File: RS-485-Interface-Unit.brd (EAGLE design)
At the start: 53.4 x 30.4 mm, 16 parts, among them IC1 B0505S, IC2 ADM2483, IC3 78L05Z, X1 RJ11CONNECTOR, X2 RJ11CONNECTOR

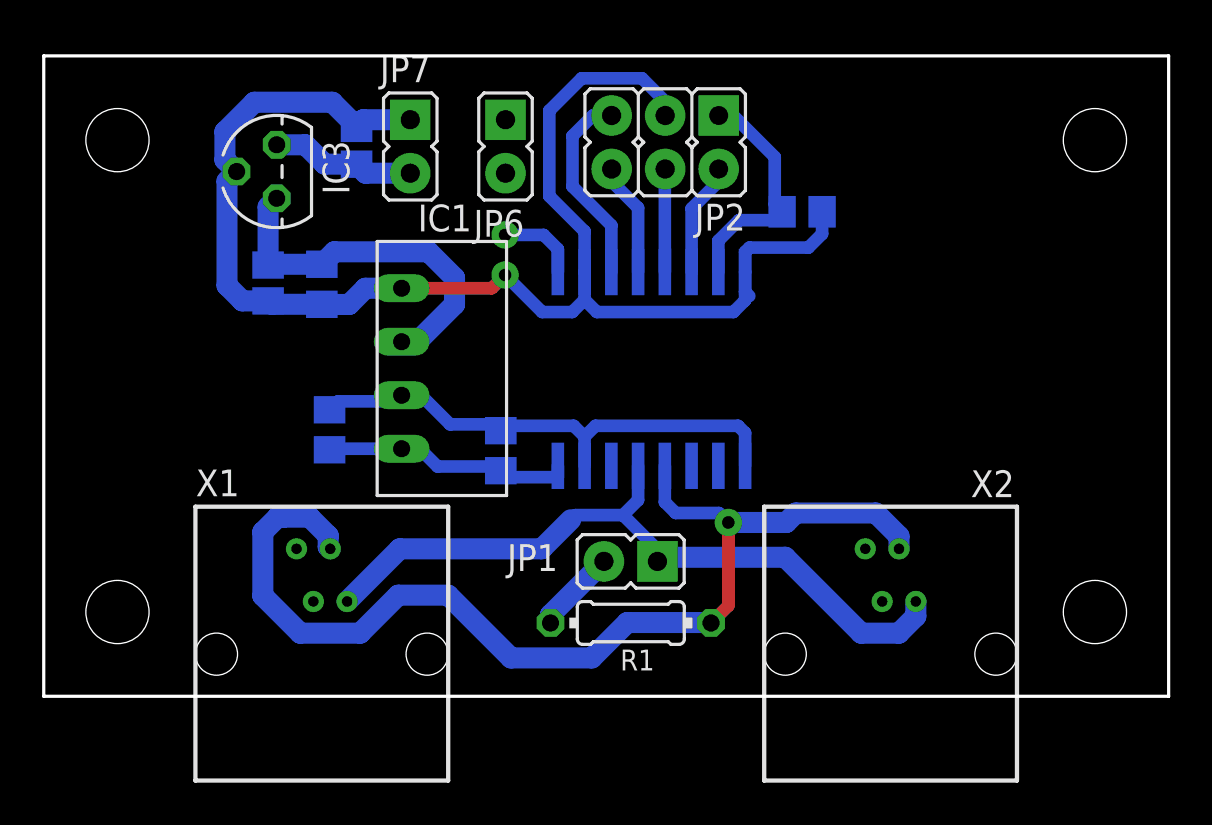
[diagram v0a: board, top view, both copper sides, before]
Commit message: Board tracing done
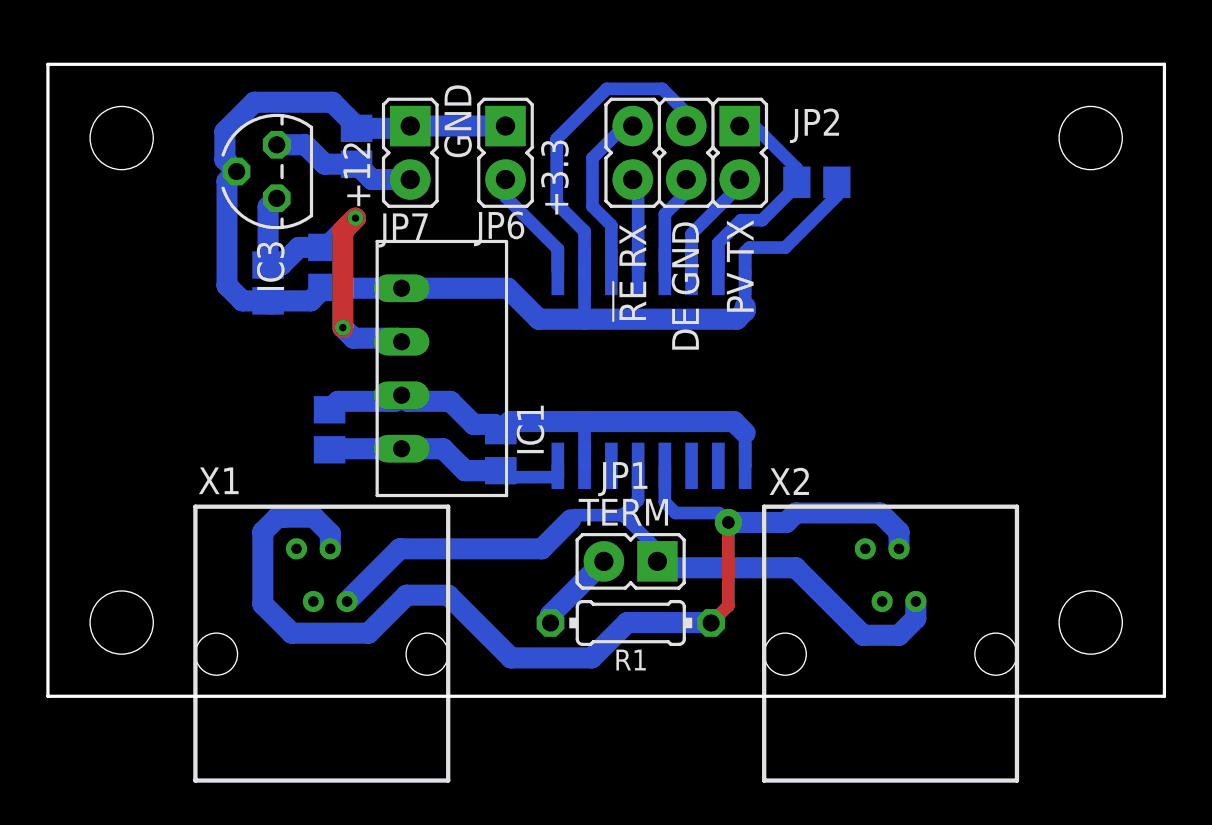
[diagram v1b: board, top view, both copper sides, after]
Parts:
- JP1: value (none) -> TERM
- moved R11 1.57 mm to (44.0, 31.0)
- moved JP2 1.12 mm to (37.8, 32.4)
- moved C2 0.81 mm to (20.6, 27.0)
- moved JP6 0.30 mm to (29.2, 32.4)
- moved JP7 0.30 mm to (24.7, 32.4)
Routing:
- net GND: track 69.4 -> 75.0 mm, vias 1 -> 0
- net VCCIO: track 12.0 -> 13.9 mm
- net +3V3: track 3.87 -> 5.42 mm, vias 1 -> 0
- net UART_RX: track 9.49 -> 8.32 mm
- net UART_TX: track 5.42 -> 6.40 mm
- net !RE: track 5.41 -> 4.50 mm
- net GNDIO: track 24.3 -> 25.1 mm
- net POWER_VALID: track 11.3 -> 10.6 mm
- net +5V: track 17.5 -> 17.0 mm, vias 0 -> 2
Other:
- board size 53.4 x 30.4 mm -> 53 x 30 mm
- board text added: "!RE! RX"
- board text added: "+12"
- board text added: "+3.3"
- board text added: "DE GND"
- board text added: "GND"
- board text added: "PV TX"
- board text added: "TERM"
